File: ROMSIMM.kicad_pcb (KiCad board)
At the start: 4 copper layers, 97.8 x 25 mm, 39 parts, among them J1 ROM, SW1 ROM Sel., U1 MX29LV640, U10 74AHC245, U11 XC6206P332MR, U12 74LVC1G02GW, U2 MX29LV640, U3 74AHC245, U4 74AHC245, U5 74AHC245, U6 74AHC245, U7 74AHC245, U9 74AHC245

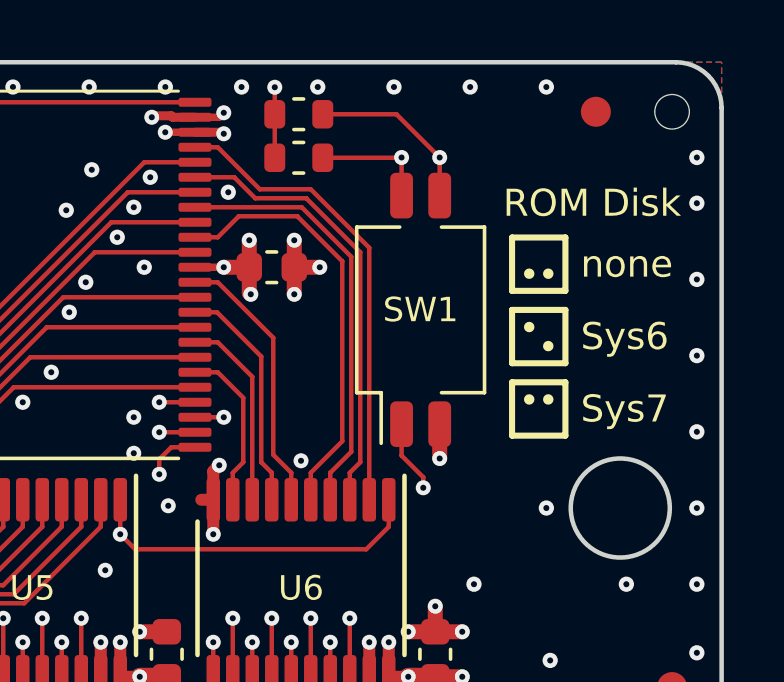
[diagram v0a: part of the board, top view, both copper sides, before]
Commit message: Start on triple DIP switch
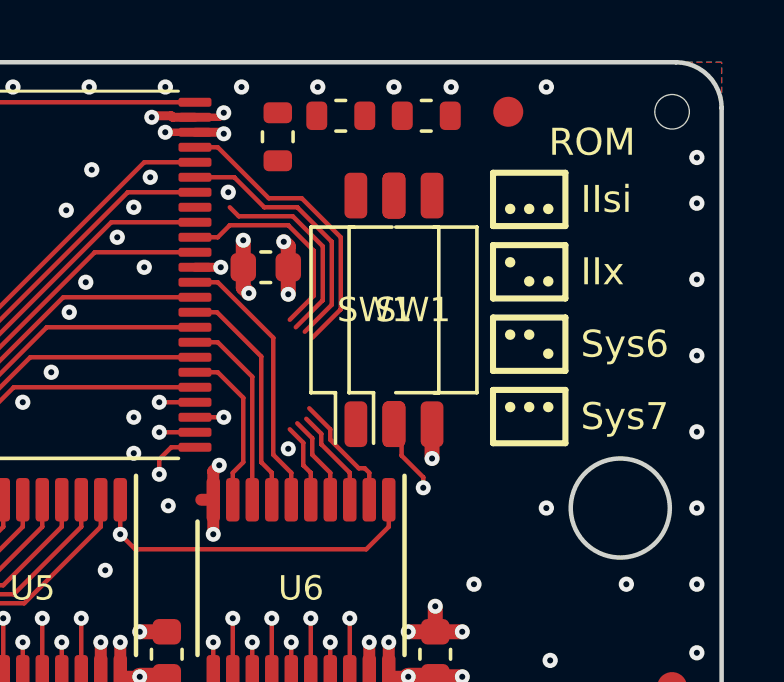
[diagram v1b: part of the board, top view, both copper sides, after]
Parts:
- added R1: 3k3, stdpads:R_0603, F.Cu at (159.7, 104.4)
- added SW1: ROM Sel., stdpads:SW_DIP_SPSTx02_Slide_DSHP02TS_P1.27mm, F.Cu at (158.0, 110.9)
- moved FID4 2.92 mm to (162.4, 104.3)
- moved R1 1.40 mm to (156.8, 104.4)
- moved R2 0.99 mm to (154.8, 105.1), turned to 90 degrees
- moved SW1 0.25 mm to (159.3, 110.9)
- moved C5 0.20 mm to (154.3, 109.5)
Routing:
- net /RA23: track 95.7 -> 89.4 mm, vias 3 -> 2
- net /RD29: track 14.3 -> 9.72 mm
- net /RD28: track 14.2 -> 9.74 mm
- net /RA22sw: track 79.4 -> 75.4 mm, vias 3 -> 2
- net +3V3: track 58.2 -> 55.0 mm, vias 75 -> 74
- net /RD30: track 14.9 -> 12.1 mm
- net /RD31: track 15.6 -> 13.8 mm
- net GND: track 84.9 -> 84.1 mm, vias 153 -> 152
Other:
- board text added: "IIsi"
- board text added: "IIx"
- board text added: "ROM"
- board text removed: "ROM Disk"
- board text removed: "none"
